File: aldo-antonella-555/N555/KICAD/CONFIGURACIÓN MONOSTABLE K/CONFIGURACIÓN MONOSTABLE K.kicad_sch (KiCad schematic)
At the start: 9 parts, among them J1 Conn_01x02_Socket, SW1 SW_SPST, U1 LM555xM

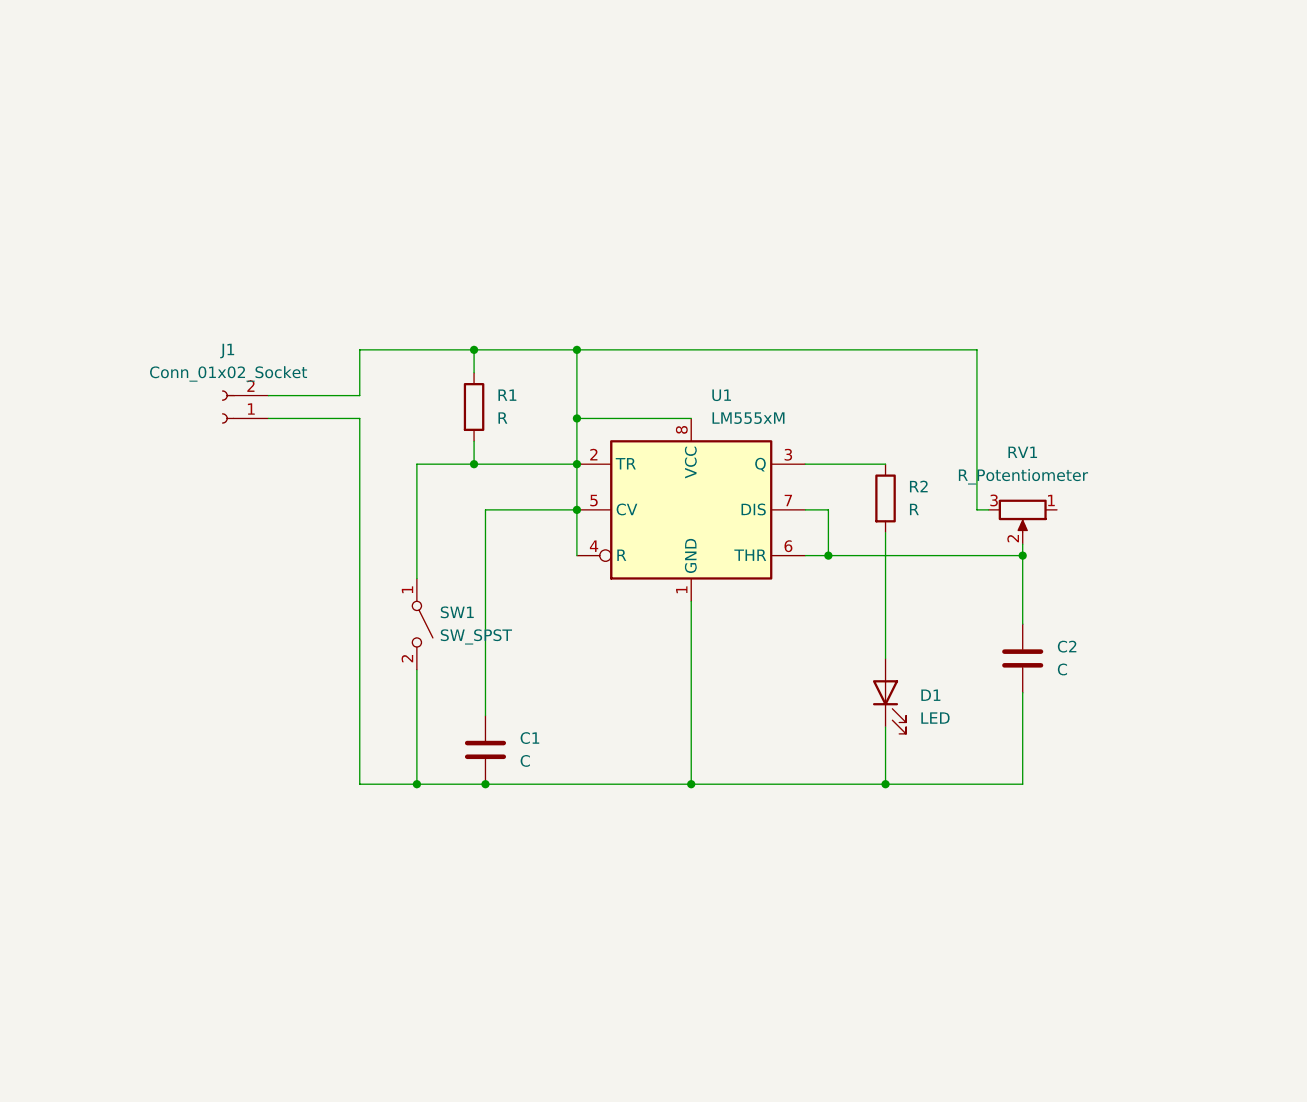
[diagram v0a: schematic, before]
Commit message: CASI FINAL
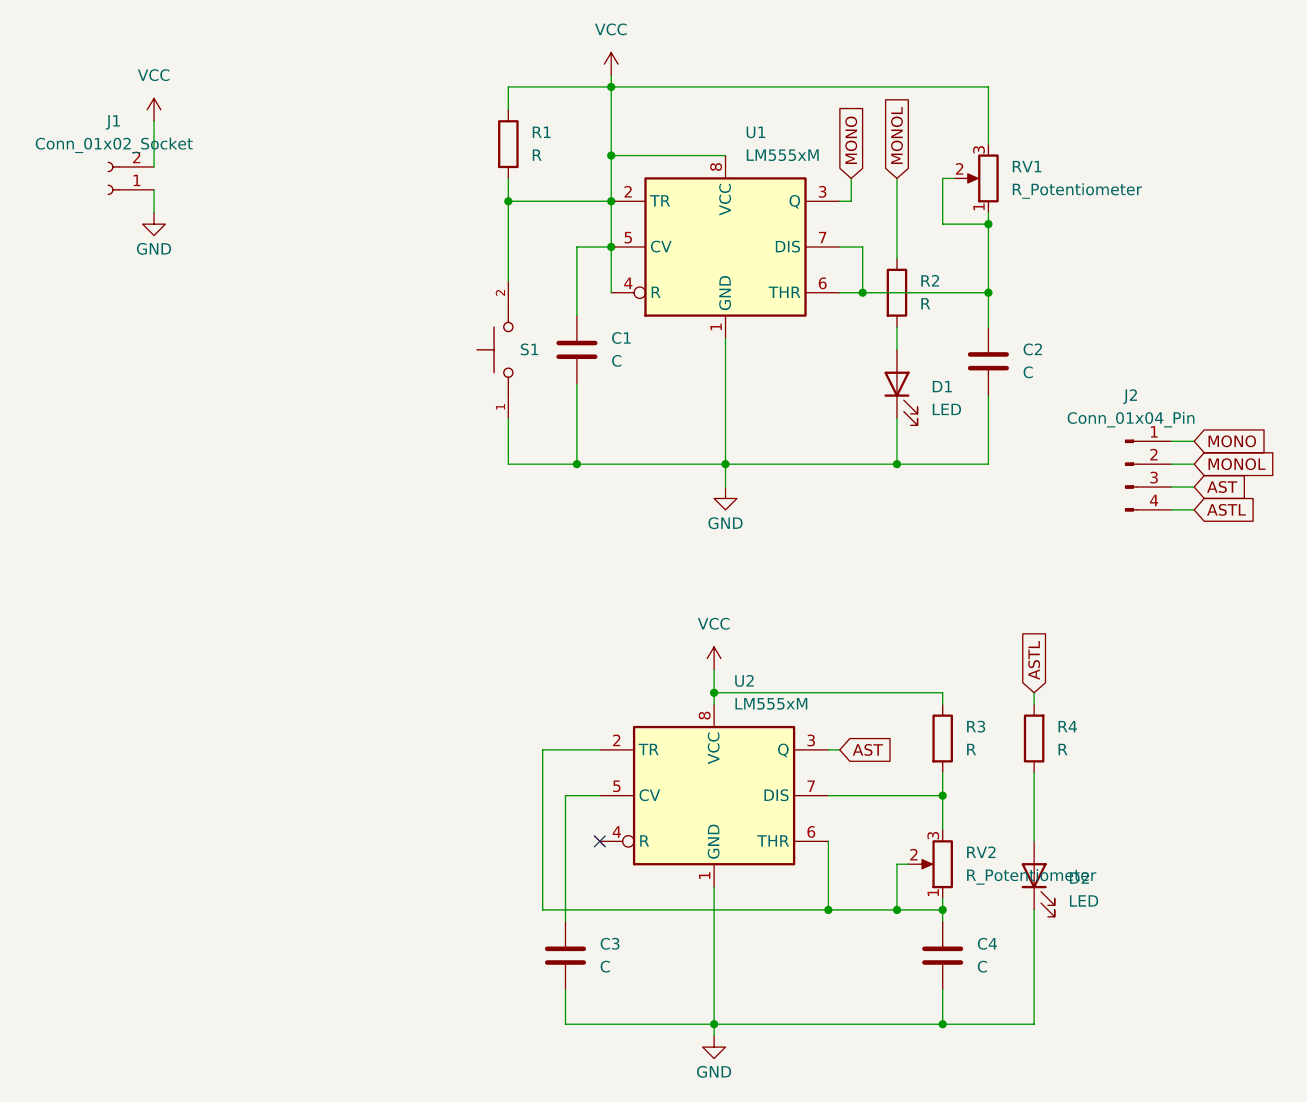
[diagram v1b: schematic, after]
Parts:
- removed SW1: SW_SPST, symbol Switch:SW_SPST
- added C3, C4: C, symbol Device:C
- added D2: LED, symbol Device:LED
- added J2: Conn_01x04_Pin, Connector_PinHeader_2.54mm:PinHeader_1x04_P2.54mm_Vertical, symbol Connector:Conn_01x04_Pin
- added R3, R4: R, symbol Device:R
- added RV2: R_Potentiometer, symbol Device:R_Potentiometer
- added S1: TL59NF160Q, TL59NF160Q:SW_TL59NF160Q, symbol TL59NF160Q:TL59NF160Q
- added U2: LM555xM, Package_SO:SOIC-8_3.9x4.9mm_P1.27mm, symbol Timer:LM555xM
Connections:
- net VCC: now reaches C1.1, J1.2 (Pin_2), R1.1, R1.2, RV1.3, U1.2 (TR), U1.4 (R), U1.5 (CV), U1.8 (VCC)
- net VCC: now also R3.1, S1.2, U2.8 (VCC)
- net GND: now reaches C1.2, C2.2, D1.1 (K), J1.1 (Pin_1), U1.1 (GND)
- net GND: now also C3.2, C4.2, D2.1 (K), S1.1, U2.1 (GND)
- net at RV1.1: now also C2.1, RV1.2, U1.6 (THR), U1.7 (DIS)
- net MONO: now reaches U1.3 (Q)
- net MONO: now also J2.1 (Pin_1); no longer R2.1
- new net: C4.1, RV2.1, RV2.2, U2.2 (TR), U2.6 (THR)
- new net: R3.2, RV2.3, U2.7 (DIS)
- new net: C3.1, U2.5 (CV)
- new net: D2.2 (A), R4.1
- new net AST: J2.3 (Pin_3), U2.3 (Q)
- new net ASTL: J2.4 (Pin_4), R4.2
- new net MONOL: J2.2 (Pin_2), R2.1
- no-connect marks 0 -> 1
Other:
- moved on the sheet: C1, C2, D1, J1, R1, R2, RV1, U1
